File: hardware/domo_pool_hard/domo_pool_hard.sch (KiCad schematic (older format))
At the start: 0 parts

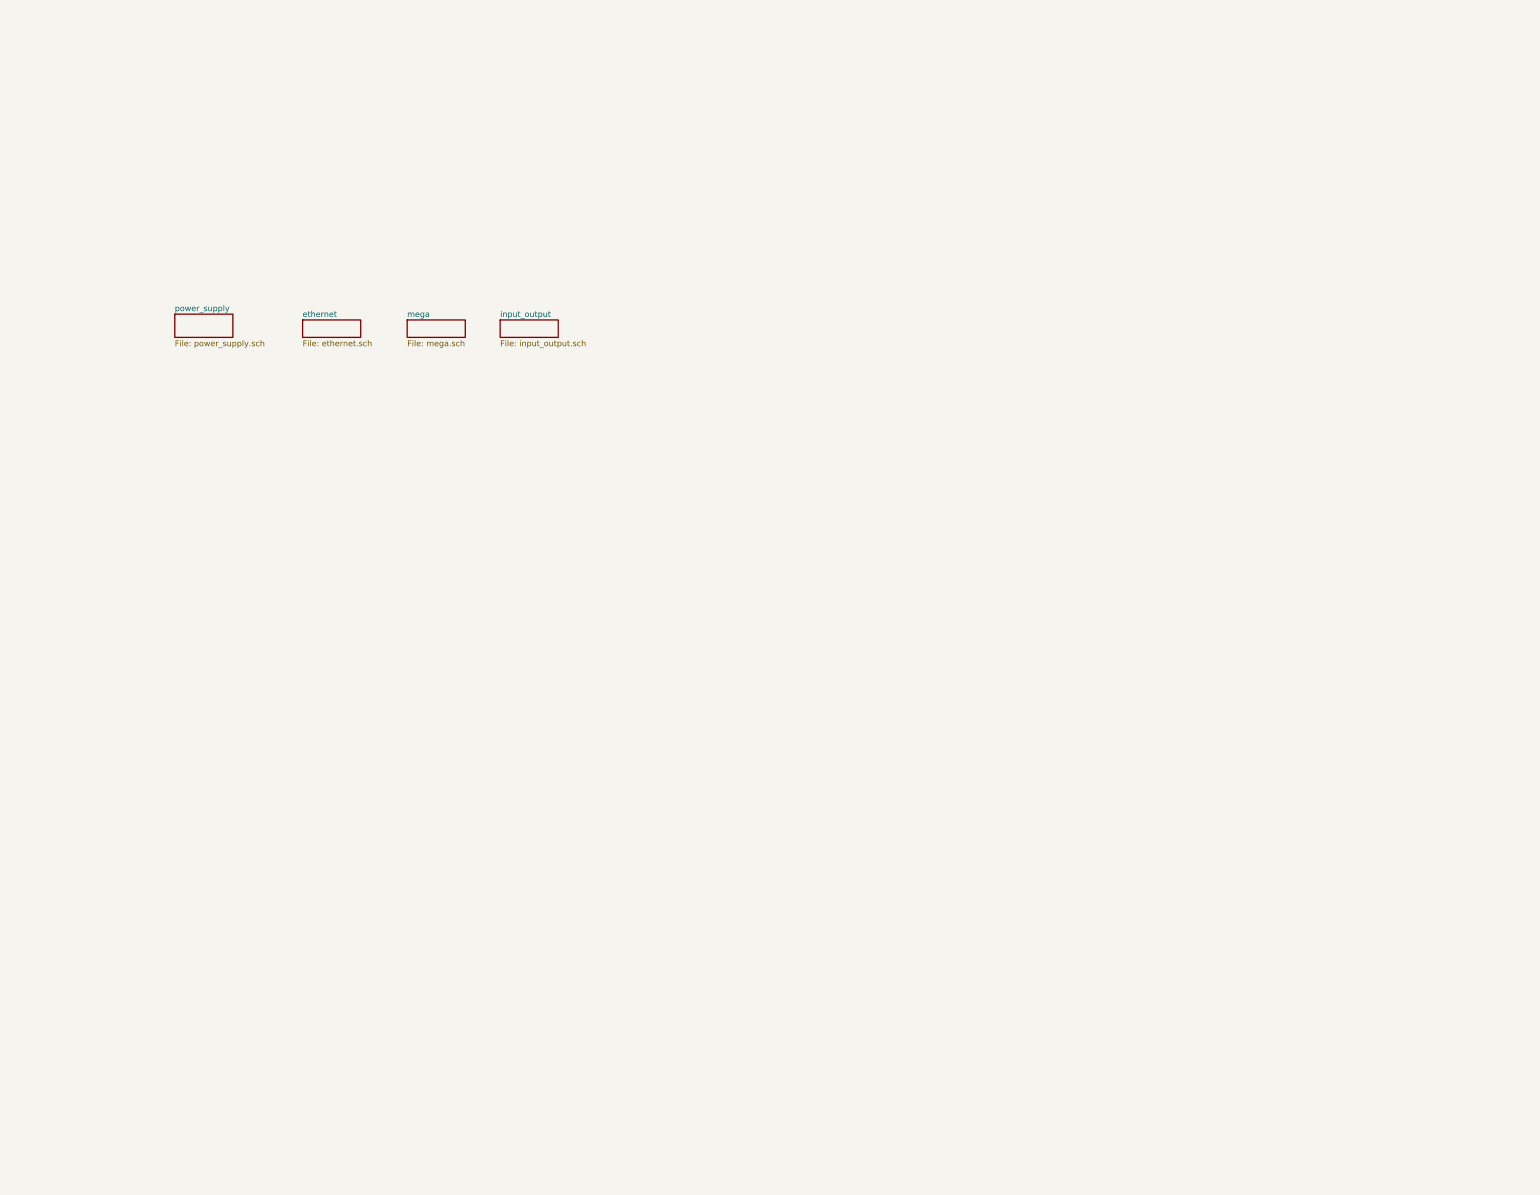
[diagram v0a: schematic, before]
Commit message: recent code + schematic
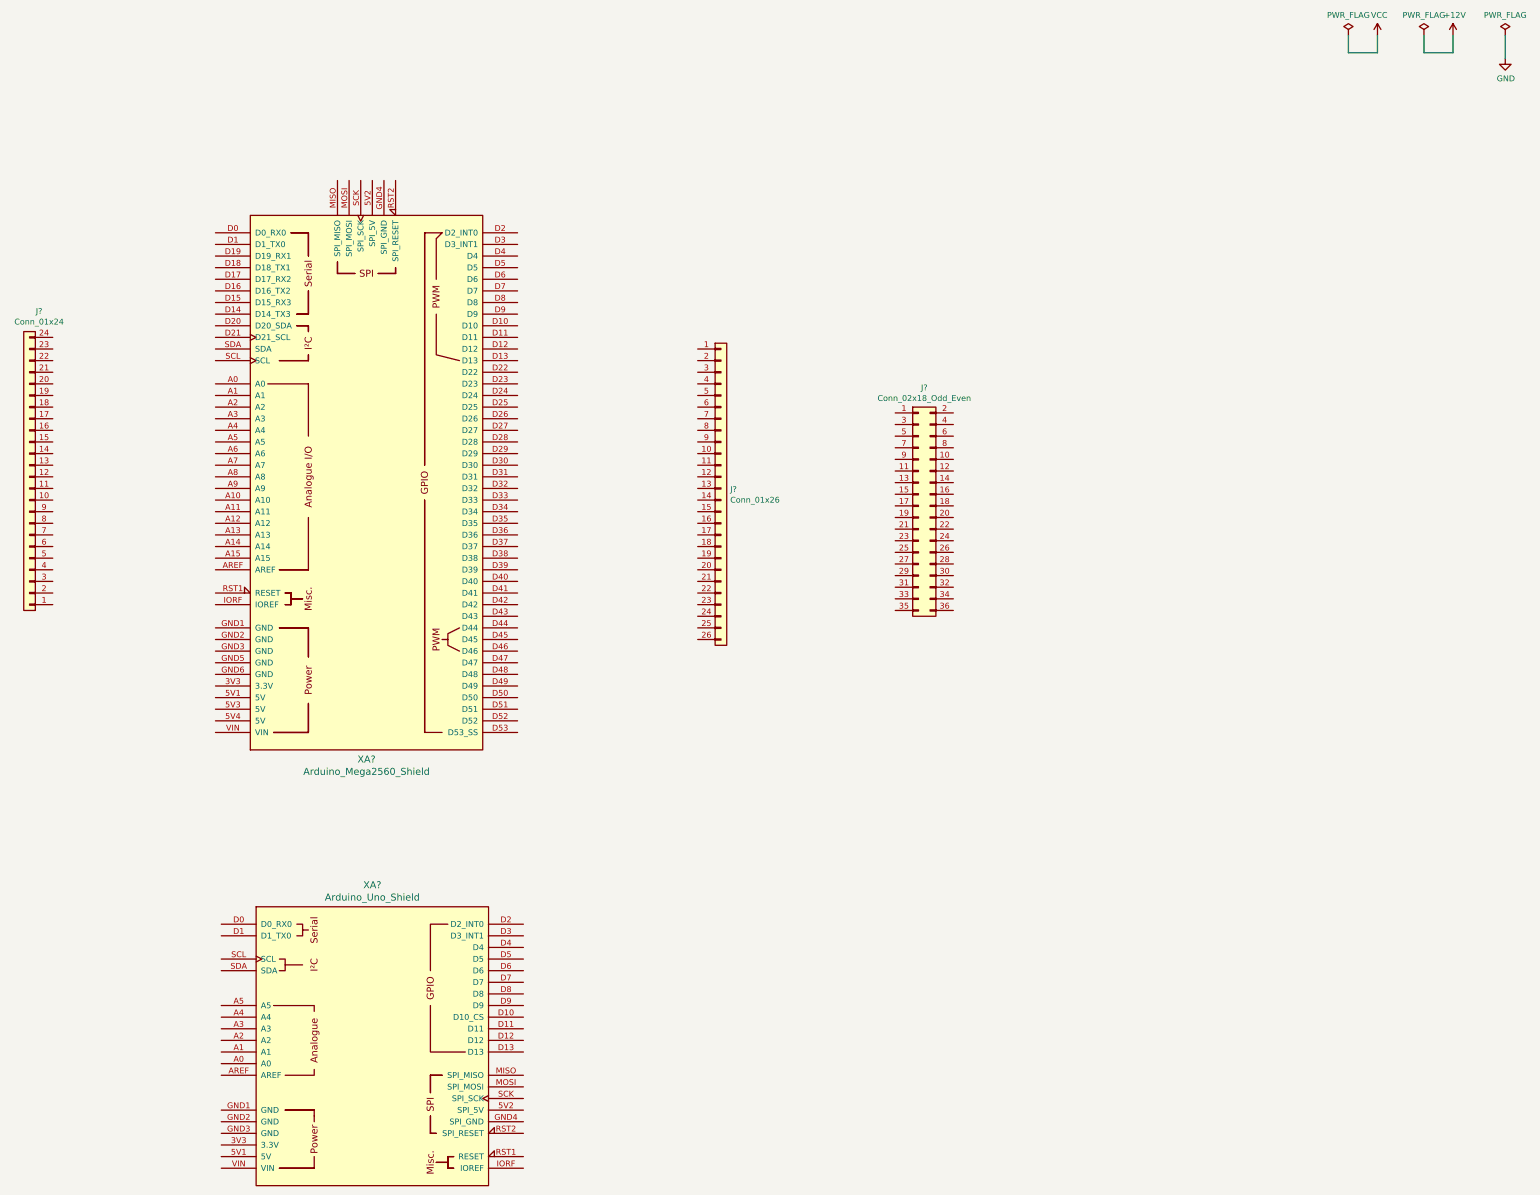
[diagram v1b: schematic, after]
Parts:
- added J?: Conn_02x18_Odd_Even, symbol Connector_Generic:Conn_02x18_Odd_Even
- added J?: Conn_01x26, symbol Connector_Generic:Conn_01x26
- added J?: Conn_01x24, symbol Connector_Generic:Conn_01x24
- added XA?: Arduino_Mega2560_Shield, symbol arduino:Arduino_Mega2560_Shield
- added XA?: Arduino_Uno_Shield, symbol arduino:Arduino_Uno_Shield
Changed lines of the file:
@@
 EESchema Schematic File Version 4
-EELAYER 29 0
+EELAYER 30 0
 EELAYER END
-$Descr A4 11693 8268
+$Descr A3 16535 11693
 encoding utf-8
-Sheet 1 4
+Sheet 1 1
 Title "Domo interface"
 Date "2020-12-06"
@@
 Comment4 ""
 $EndDescr
-$Sheet
-S 5150 3400 500  150
-U 5FCDB50C
-F0 "ethernet" 50
-F1 "ethernet.sch" 50
-$EndSheet
-$Sheet
-S 4050 3350 500  200
-U 5FCDBA1F
-F0 "power_supply" 50
-F1 "power_supply.sch" 50
-$EndSheet
-$Sheet
-S 6050 3400 500  150
-U 5FCDDB53
-F0 "mega" 50
-F1 "mega.sch" 50
-$EndSheet
-$Sheet
-S 6850 3400 500  150
-U 5FCE2868
-F0 "input_output" 50
-F1 "input_output.sch" 50
-$EndSheet
+$Comp
+L arduino:Arduino_Mega2560_Shield XA?
+U 1 1 6103D51B
+P 5700 4800
+F 0 "XA?" H 5700 2419 60  0000 C CNN
+F 1 "Arduino_Mega2560_Shield" H 5700 2313 60  0000 C CNN
+F 2 "" H 6400 7550 60  0001 C CNN
+F 3 "https://store.arduino.cc/arduino-mega-2560-rev3" H 6400 7550 60  0001 C CNN
+	1    5700 4800
+	1    0    0    -1
+$EndComp
+$Comp
+L arduino:Arduino_Uno_Shield XA?
+U 1 1 61043145
+P 5750 9650
+F 0 "XA?" H 5750 11037 60  0000 C CNN
+F 1 "Arduino_Uno_Shield" H 5750 10931 60  0000 C CNN
+F 2 "" H 7550 13400 60  0001 C CNN
+F 3 "https://store.arduino.cc/arduino-uno-rev3" H 7550 13400 60  0001 C CNN
+	1    5750 9650
+	1    0    0    -1
+$EndComp
+$Comp
+L Connector_Generic:Conn_02x18_Odd_Even J?
+U 1 1 6107FDB2
+P 10450 5000
+F 0 "J?" H 10500 6017 50  0000 C CNN
+F 1 "Conn_02x18_Odd_Even" H 10500 5926 50  0000 C CNN
+F 2 "" H 10450 5000 50  0001 C CNN
+F 3 "~" H 10450 5000 50  0001 C CNN
+	1    10450 5000
+	1    0    0    -1
+$EndComp
+$Comp
+L Connector_Generic:Conn_01x26 J?
+U 1 1 61090DBA
+P 8750 4850
+F 0 "J?" H 8830 4842 50  0000 L CNN
+F 1 "Conn_01x26" H 8830 4751 50  0000 L CNN
+F 2 "" H 8750 4850 50  0001 C CNN
+F 3 "~" H 8750 4850 50  0001 C CNN
+	1    8750 4850
+	1    0    0    -1
+$EndComp
+$Comp
+L Connector_Generic:Conn_01x24 J?
+U 1 1 610B5E9E
+P 2800 4750
+F 0 "J?" H 2718 3325 50  0000 C CNN
+F 1 "Conn_01x24" H 2718 3416 50  0000 C CNN
+F 2 "" H 2800 4750 50  0001 C CNN
+F 3 "~" H 2800 4750 50  0001 C CNN
+	1    2800 4750
+	-1   0    0    1
+$EndComp
+$Comp
+L power:PWR_FLAG #FLG?
+U 1 1 610CD1B2
+P 14150 950
+F 0 "#FLG?" H 14150 1025 50  0001 C CNN
+F 1 "PWR_FLAG" H 14150 1123 50  0000 C CNN
+F 2 "" H 14150 950 50  0001 C CNN
+F 3 "~" H 14150 950 50  0001 C CNN
+	1    14150 950
+	1    0    0    -1
+$EndComp
+$Comp
+L power:PWR_FLAG #FLG?
+U 1 1 610CE480
+P 14800 950
+F 0 "#FLG?" H 14800 1025 50  0001 C CNN
+F 1 "PWR_FLAG" H 14800 1123 50  0000 C CNN
+F 2 "" H 14800 950 50  0001 C CNN
+F 3 "~" H 14800 950 50  0001 C CNN
+	1    14800 950
+	1    0    0    -1
+$EndComp
+$Comp
+L power:PWR_FLAG #FLG?
+U 1 1 610CE6E2
+P 15500 950
+F 0 "#FLG?" H 15500 1025 50  0001 C CNN
+F 1 "PWR_FLAG" H 15500 1123 50  0000 C CNN
+F 2 "" H 15500 950 50  0001 C CNN
+F 3 "~" H 15500 950 50  0001 C CNN
+	1    15500 950
+	1    0    0    -1
+$EndComp
+$Comp
+L power:VCC #PWR?
+U 1 1 610CE9BC
+P 14400 950
+F 0 "#PWR?" H 14400 800 50  0001 C CNN
+F 1 "VCC" H 14415 1123 50  0000 C CNN
+F 2 "" H 14400 950 50  0001 C CNN
+F 3 "" H 14400 950 50  0001 C CNN
+	1    14400 950
+	1    0    0    -1
+$EndComp
+$Comp
+L power:+12V #PWR?
+U 1 1 610CEE51
+P 15050 950
+F 0 "#PWR?" H 15050 800 50  0001 C CNN
+F 1 "+12V" H 15065 1123 50  0000 C CNN
+F 2 "" H 15050 950 50  0001 C CNN
+F 3 "" H 15050 950 50  0001 C CNN
+	1    15050 950
+	1    0    0    -1
+$EndComp
+$Comp
+L power:GND #PWR?
+U 1 1 610CF26B
+P 15500 1150
+F 0 "#PWR?" H 15500 900 50  0001 C CNN
+F 1 "GND" H 15505 977 50  0000 C CNN
+F 2 "" H 15500 1150 50  0001 C CNN
+F 3 "" H 15500 1150 50  0001 C CNN
+	1    15500 1150
+	1    0    0    -1
+$EndComp
+Wire Wire Line
+	15500 950  15500 1150
+Wire Wire Line
+	15050 950  15050 1100
+Wire Wire Line
+	15050 1100 14800 1100
+Wire Wire Line
+	14800 1100 14800 950
+Wire Wire Line
+	14400 950  14400 1100
+Wire Wire Line
+	14400 1100 14150 1100
+Wire Wire Line
+	14150 1100 14150 950
 $EndSCHEMATC

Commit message: schematic
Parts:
- added C? (x2): C, symbol Device:C
- added J? (x3): Screw_Terminal_01x08, symbol Connector:Screw_Terminal_01x08
- added J? (x2): Conn_02x09_Odd_Even, symbol Connector_Generic:Conn_02x09_Odd_Even
- added J? (x2): Screw_Terminal_01x02, symbol Connector:Screw_Terminal_01x02
- added J?: Screw_Terminal_01x11, symbol Connector:Screw_Terminal_01x11
- added J?: Screw_Terminal_01x12, symbol Connector:Screw_Terminal_01x12
- added J?: Screw_Terminal_01x04, symbol Connector:Screw_Terminal_01x04
- added U? (x2): TCA9555DBR, Package_SO:SSOP-24_5.3x8.2mm_P0.65mm, symbol Interface_Expansion:TCA9555DBR
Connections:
- net +12V: now also J?.1 (Pin_1), J?.2 (Pin_2)
- net GND: now also J?.18 (Pin_18), J?.19 (Pin_19), J?.35 (Pin_35), J?.36 (Pin_36), J?.4 (Pin_4), XA?.GND1 (GND), XA?.GND1 (GND), XA?.GND2 (GND), XA?.GND2 (GND), XA?.GND3 (GND), XA?.GND3 (GND), XA?.GND5 (GND), XA?.GND6 (GND), C?.2, C?.2, J?.1 (Pin_1), J?.11 (Pin_11), J?.12 (Pin_12), J?.17 (Pin_17), J?.17 (Pin_17), J?.18 (Pin_18), J?.18 (Pin_18), J?.2 (Pin_2), J?.3 (Pin_3), J?.4 (Pin_4), J?.5 (Pin_5), J?.6 (Pin_6), J?.7 (Pin_7), J?.8 (Pin_8), U?.12 (GND), U?.12 (GND), U?.2 (A1), U?.21 (A0), U?.3 (A2)
- net VCC: now also J?.1 (Pin_1), J?.17 (Pin_17), J?.2 (Pin_2), J?.20 (Pin_20), J?.23 (Pin_23), XA?.5V1 (5V), XA?.5V1 (5V), XA?.5V3 (5V), XA?.5V4 (5V), XA?.VIN, XA?.VIN, C?.1, C?.1, J?.1 (Pin_1), J?.1 (Pin_1), J?.1 (Pin_1), J?.2 (Pin_2), J?.2 (Pin_2), J?.2 (Pin_2), J?.3 (Pin_3), J?.3 (Pin_3), J?.4 (Pin_4), J?.4 (Pin_4), U?.2 (A1), U?.21 (A0), U?.24 (VCC), U?.24 (VCC), U?.3 (A2)
- net 3v3: now reaches XA?.3V3 (3.3V)
- net 3v3: now also J?.21 (Pin_21), XA?.3V3 (3.3V)
- net spi5v: now reaches XA?.5V2 (SPI_5V)
- net spi5v: now also XA?.5V2 (SPI_5V)
- net A0: now reaches XA?.A0
- net A0: now also J?.16 (Pin_16), XA?.A0, J?.8 (Pin_8)
- net A1: now reaches XA?.A1
- net A1: now also J?.15 (Pin_15), XA?.A1, J?.7 (Pin_7)
- net A10: now reaches XA?.A10
- net A10: now also J?.6 (Pin_6)
- net A11: now reaches XA?.A11
- net A11: now also J?.5 (Pin_5)
- net A12: now reaches XA?.A12
- net A12: now also J?.4 (Pin_4)
- net A13: now reaches XA?.A13
- net A13: now also J?.3 (Pin_3)
- net A14: now reaches XA?.A14
- net A14: now also J?.2 (Pin_2)
- net A15: now reaches XA?.A15
- net A15: now also J?.1 (Pin_1)
- net A2: now reaches XA?.A2
- net A2: now also J?.14 (Pin_14), XA?.A2, J?.6 (Pin_6)
- net A3: now reaches XA?.A3
- net A3: now also J?.13 (Pin_13), XA?.A3, J?.5 (Pin_5)
- net A4: now reaches XA?.A4
- net A4: now also J?.12 (Pin_12), XA?.A4, J?.4 (Pin_4)
- net A5: now reaches XA?.A5
- net A5: now also J?.11 (Pin_11), XA?.A5, J?.3 (Pin_3)
- net A6: now reaches XA?.A6
- net A6: now also J?.10 (Pin_10), J?.2 (Pin_2)
- net A7: now reaches XA?.A7
- net A7: now also J?.9 (Pin_9), J?.1 (Pin_1)
- net A8: now reaches XA?.A8
- net A8: now also J?.8 (Pin_8)
- net A9: now reaches XA?.A9
- net A9: now also J?.7 (Pin_7)
- net Aref: now reaches XA?.AREF
- net Aref: now also J?.3 (Pin_3), XA?.AREF
- net 0: now reaches XA?.D0 (D0_RX0)
- net 0: now also J?.18 (Pin_18), XA?.D0 (D0_RX0)
- net 1: now reaches XA?.D1 (D1_TX0)
- net 1: now also J?.17 (Pin_17), XA?.D1 (D1_TX0)
- net 10: now reaches XA?.D10
- net 10: now also J?.8 (Pin_8), XA?.D10 (D10_CS), J?.9 (Pin_9)
- net 11: now reaches XA?.D11
- net 11: now also J?.7 (Pin_7), XA?.D11, J?.10 (Pin_10)
- net 12: now reaches XA?.D12
- net 12: now also J?.6 (Pin_6), XA?.D12, J?.11 (Pin_11)
- net 13: now reaches XA?.D13
- net 13: now also J?.5 (Pin_5), XA?.D13
- net 14: now reaches XA?.D14 (D14_TX3)
- net 14: now also J?.19 (Pin_19)
- net 15: now reaches XA?.D15 (D15_RX3)
- net 15: now also J?.20 (Pin_20)
- net 16: now reaches XA?.D16 (D16_TX2)
- net 16: now also J?.21 (Pin_21)
- net 17: now reaches XA?.D17 (D17_RX2)
- net 17: now also J?.22 (Pin_22)
- net 18: now reaches XA?.D18 (D18_TX1)
- net 18: now also J?.23 (Pin_23)
- net 19: now reaches XA?.D19 (D19_RX1)
- net 19: now also J?.24 (Pin_24)
- net 2: now reaches XA?.D2 (D2_INT0)
- net 2: now also J?.16 (Pin_16), XA?.D2 (D2_INT0), J?.1 (Pin_1)
- net 20: now reaches XA?.D20 (D20_SDA)
- net 20: now also J?.25 (Pin_25)
- net 21: now reaches XA?.D21 (D21_SCL)
- net 21: now also J?.26 (Pin_26)
- net 22: now reaches XA?.D22
- net 22: now also J?.3 (Pin_3)
- net 23: now reaches XA?.D23
- net 23: now also J?.4 (Pin_4)
- net 24: now reaches XA?.D24
- net 24: now also J?.5 (Pin_5)
- net 25: now reaches XA?.D25
- net 25: now also J?.6 (Pin_6)
- net 26: now reaches XA?.D26
- net 26: now also J?.7 (Pin_7)
- net 27: now reaches XA?.D27
- net 27: now also J?.8 (Pin_8)
- net 28: now reaches XA?.D28
- net 28: now also J?.9 (Pin_9)
- net 29: now reaches XA?.D29
- net 29: now also J?.10 (Pin_10)
- net 3: now reaches XA?.D3 (D3_INT1)
- net 3: now also J?.15 (Pin_15), XA?.D3 (D3_INT1), J?.2 (Pin_2)
- net 30: now reaches XA?.D30
- net 30: now also J?.11 (Pin_11)
- net 31: now reaches XA?.D31
- net 31: now also J?.12 (Pin_12)
- net 32: now reaches XA?.D32
- net 32: now also J?.13 (Pin_13)
- net 33: now reaches XA?.D33
- net 33: now also J?.14 (Pin_14)
- net 34: now reaches XA?.D34
- net 34: now also J?.15 (Pin_15)
- net 35: now reaches XA?.D35
- net 35: now also J?.16 (Pin_16)
- net 36: now reaches XA?.D36
- net 36: now also J?.17 (Pin_17)
- net 37: now reaches XA?.D37
- net 37: now also J?.18 (Pin_18)
- net 38: now reaches XA?.D38
- net 38: now also J?.19 (Pin_19)
- net 39: now reaches XA?.D39
- net 39: now also J?.20 (Pin_20)
- net 4: now reaches XA?.D4
- net 4: now also J?.14 (Pin_14), XA?.D4, J?.3 (Pin_3)
- net 40: now reaches XA?.D40
- net 40: now also J?.21 (Pin_21)
- net 41: now reaches XA?.D41
- net 41: now also J?.22 (Pin_22)
- net 42: now reaches XA?.D42
- net 42: now also J?.23 (Pin_23)
- net 43: now reaches XA?.D43
- net 43: now also J?.24 (Pin_24)
- net 44: now reaches XA?.D44
- net 44: now also J?.25 (Pin_25), J?.1 (Pin_1)
- net 45: now reaches XA?.D45
- net 45: now also J?.26 (Pin_26), J?.2 (Pin_2)
- net 46: now reaches XA?.D46
- net 46: now also J?.27 (Pin_27), J?.3 (Pin_3)
- net 47: now reaches XA?.D47
- net 47: now also J?.28 (Pin_28), J?.4 (Pin_4)
- net 48: now reaches XA?.D48
- net 48: now also J?.29 (Pin_29), J?.5 (Pin_5)
- net 49: now reaches XA?.D49
- net 49: now also J?.30 (Pin_30), J?.6 (Pin_6)
- net 5: now reaches XA?.D5
- net 5: now also J?.13 (Pin_13), XA?.D5, J?.4 (Pin_4)
- net 50: now reaches XA?.D50
- net 50: now also J?.31 (Pin_31), J?.7 (Pin_7)
- net 51: now reaches XA?.D51
- net 51: now also J?.32 (Pin_32), J?.8 (Pin_8)
- net 52: now reaches XA?.D52
- net 52: now also J?.33 (Pin_33), J?.9 (Pin_9)
- net 53: now reaches XA?.D53 (D53_SS)
- net 53: now also J?.34 (Pin_34), J?.10 (Pin_10)
- net 6: now reaches XA?.D6
- net 6: now also J?.12 (Pin_12), XA?.D6, J?.5 (Pin_5)
- net 7: now reaches XA?.D7
- net 7: now also J?.11 (Pin_11), XA?.D7, J?.6 (Pin_6)
- net 8: now reaches XA?.D8
- net 8: now also J?.10 (Pin_10), XA?.D8, J?.7 (Pin_7)
- net 9: now reaches XA?.D9
- net 9: now also J?.9 (Pin_9), XA?.D9, J?.8 (Pin_8)
- net spignd: now reaches XA?.GND4 (SPI_GND)
- net spignd: now also XA?.GND4 (SPI_GND)
- net ioref: now reaches XA?.IORF (IOREF)
- net ioref: now also XA?.IORF (IOREF)
- net miso: now reaches XA?.MISO (SPI_MISO)
- net miso: now also XA?.MISO (SPI_MISO)
- net mosi: now reaches XA?.MOSI (SPI_MOSI)
- net mosi: now also XA?.MOSI (SPI_MOSI)
- net RST: now reaches XA?.RST1 (RESET)
- net RST: now also J?.22 (Pin_22), XA?.RST1 (RESET)
- net spi_res: now reaches XA?.RST2 (SPI_RESET)
- net spi_res: now also XA?.RST2 (SPI_RESET)
- net sck: now reaches XA?.SCK (SPI_SCK)
- net sck: now also XA?.SCK (SPI_SCK)
- net scl: now reaches XA?.SCL
- net scl: now also J?.1 (Pin_1), XA?.SCL, U?.22 (SCL), U?.22 (SCL)
- net sda: now reaches XA?.SDA
- net sda: now also J?.2 (Pin_2), XA?.SDA, U?.23 (SDA), U?.23 (SDA)
- new net: J?.5 (Pin_5), J?.6 (Pin_6), J?.7 (Pin_7), J?.8 (Pin_8)
- new net: J?.7 (Pin_7), U?.10 (P06) (x2)
- new net: J?.8 (Pin_8), U?.11 (P07) (x2)
- new net: J?.9 (Pin_9), U?.13 (P10) (x2)
- new net: J?.10 (Pin_10), U?.14 (P11) (x2)
- new net: J?.11 (Pin_11), U?.15 (P12) (x2)
- new net: J?.12 (Pin_12), U?.16 (P13) (x2)
- new net: J?.13 (Pin_13), U?.17 (P14) (x2)
- new net: J?.14 (Pin_14), U?.18 (P15) (x2)
- new net: J?.15 (Pin_15), U?.19 (P16) (x2)
- new net: J?.16 (Pin_16), U?.20 (P17) (x2)
- new net: J?.1 (Pin_1), U?.4 (P00) (x2)
- new net: J?.2 (Pin_2), U?.5 (P01) (x2)
- new net: J?.3 (Pin_3), U?.6 (P02) (x2)
- new net: J?.4 (Pin_4), U?.7 (P03) (x2)
- new net: J?.5 (Pin_5), U?.8 (P04) (x2)
- new net: J?.6 (Pin_6), U?.9 (P05) (x2)
- no-connect marks 0 -> 3
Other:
- moved on the sheet: J?, XA?

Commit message: schematic power...
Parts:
- removed J?: Screw_Terminal_01x04, symbol Connector:Screw_Terminal_01x04
- removed XA?: Arduino_Uno_Shield, symbol arduino:Arduino_Uno_Shield
- added C1, C2: C, symbol Device:C
- added D1, D2: D, symbol Device:D
- added J1, J5, J6: Screw_Terminal_01x02, symbol Connector:Screw_Terminal_01x02
- added J8: Screw_Terminal_01x08, symbol Connector:Screw_Terminal_01x08
- added Q1, Q2: TIP120, Package_TO_SOT_THT:TO-220-3_Vertical, symbol Transistor_BJT:TIP120
- added R1, R2: R, symbol Device:R
- added U1: MP2307mod, symbol MP2307:MP2307mod
- gave numbers to parts that had none: 17
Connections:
- net +12V: now also C1.1, C2.1, D1.1 (K), D2.1 (K), J1.1 (Pin_1), J5.1 (Pin_1), J6.1 (Pin_1), J8.1 (Pin_1), J8.2 (Pin_2), J8.3 (Pin_3), J8.4 (Pin_4), U1.2 (In+)
- net 34: now also R1.2
- net 35: now also R2.2
- net GND: now also J1.2 (Pin_2), J8.5 (Pin_5), J8.6 (Pin_6), J8.7 (Pin_7), J8.8 (Pin_8), Q1.3 (E), Q2.3 (E), U1.1 (In-), U1.3 (Out-)
- net VCC: now also U1.4 (Out+)
- new net: Q1.1 (B), R1.1
- new net: C1.2, D1.2 (A), J5.2 (Pin_2), Q1.2 (C)
- new net: Q2.1 (B), R2.1
- new net: C2.2, D2.2 (A), J6.2 (Pin_2), Q2.2 (C)
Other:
- moved on the sheet: C3, C4, J10, J11, J12, J13, J14, J15, J16, J2, J3, J4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

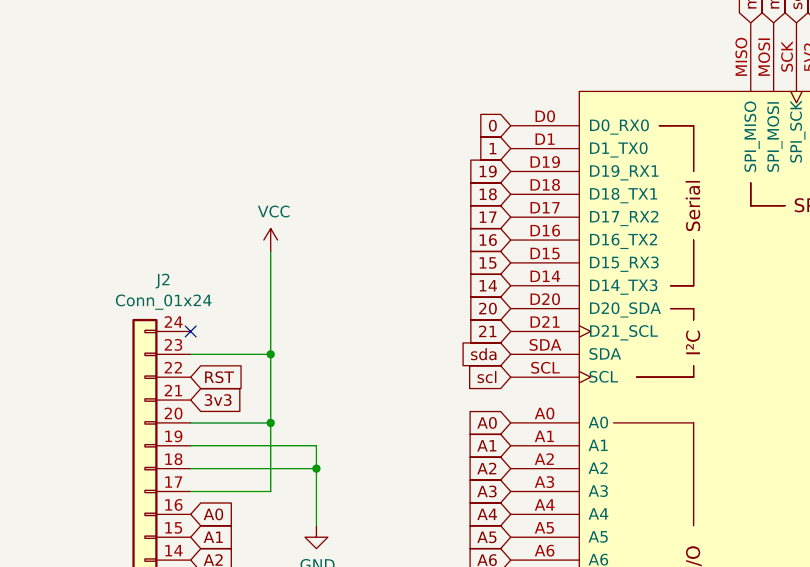
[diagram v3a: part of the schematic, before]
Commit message: schematic power...
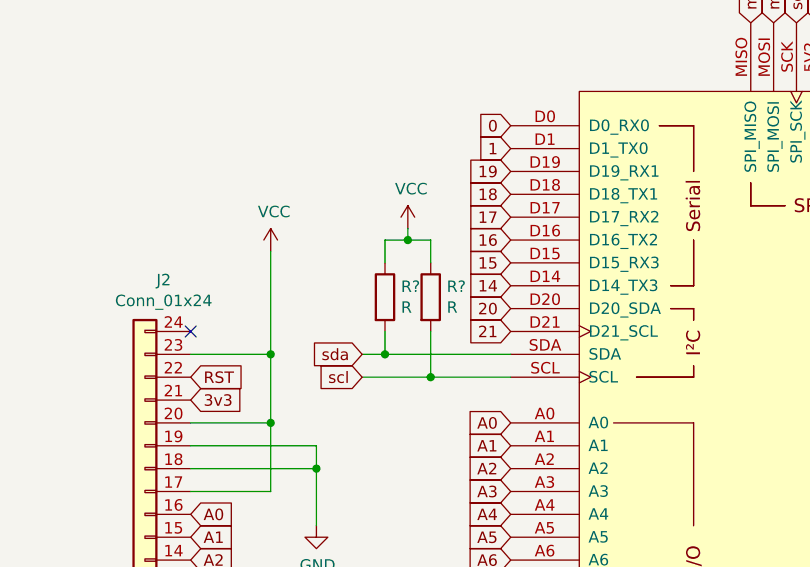
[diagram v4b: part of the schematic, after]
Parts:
- added R? (x2): R, symbol Device:R
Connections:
- net VCC: now also R?.1, R?.1
- net scl: now also R?.2
- net sda: now also R?.2
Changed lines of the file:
@@
 Text GLabel 3250 4150 0    50   Input ~ 0
 21
-Text GLabel 3250 4250 0    50   Input ~ 0
+Text GLabel 2600 4250 0    50   Input ~ 0
 sda
-Text GLabel 3250 4350 0    50   Input ~ 0
+Text GLabel 2600 4350 0    50   Input ~ 0
 scl
 Text GLabel 3250 4550 0    50   Input ~ 0
@@
 Wire Wire Line
 	6450 1300 6450 1200
+$Comp
+L Device:R R?
+U 1 1 6191D99F
+P 2700 4000
+F 0 "R?" H 2770 4046 50  0000 L CNN
+F 1 "R" H 2770 3955 50  0000 L CNN
+F 2 "" V 2630 4000 50  0001 C CNN
+F 3 "~" H 2700 4000 50  0001 C CNN
+	1    2700 4000
+	1    0    0    -1
+$EndComp
+$Comp
+L Device:R R?
+U 1 1 6191E324
+P 2900 4000
+F 0 "R?" H 2970 4046 50  0000 L CNN
+F 1 "R" H 2970 3955 50  0000 L CNN
+F 2 "" V 2830 4000 50  0001 C CNN
+F 3 "~" H 2900 4000 50  0001 C CNN
+	1    2900 4000
+	1    0    0    -1
+$EndComp
+Wire Wire Line
+	2600 4250 2700 4250
+Wire Wire Line
+	3250 4350 2900 4350
+Wire Wire Line
+	2700 4150 2700 4250
+Connection ~ 2700 4250
+Wire Wire Line
+	2700 4250 3250 4250
+Wire Wire Line
+	2900 4150 2900 4350
+Connection ~ 2900 4350
+Wire Wire Line
+	2900 4350 2600 4350
+$Comp
+L power:VCC #PWR?
+U 1 1 61988482
+P 2800 3700
+F 0 "#PWR?" H 2800 3550 50  0001 C CNN
+F 1 "VCC" H 2815 3873 50  0000 C CNN
+F 2 "" H 2800 3700 50  0001 C CNN
+F 3 "" H 2800 3700 50  0001 C CNN
+	1    2800 3700
+	1    0    0    -1
+$EndComp
+Wire Wire Line
+	2900 3850 2900 3750
+Wire Wire Line
+	2900 3750 2800 3750
+Wire Wire Line
+	2800 3750 2800 3700
+Wire Wire Line
+	2700 3850 2700 3750
+Wire Wire Line
+	2700 3750 2800 3750
+Connection ~ 2800 3750
 $EndSCHEMATC
